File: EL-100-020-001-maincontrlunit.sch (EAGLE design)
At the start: 56 parts, among them T1 WS-TST-90°, U1 VNI4140K-32, U16 24AA256-I/SN, U19 ABS10-32.768KHZ-7-T, U2 VNI4140K-32, U8 MCP7940N-I/SN, U9 PMEG2005ET, X1 944-12-46-00, X2 944-12-46-00, X3 90G-14

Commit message: DIN-rail-controller
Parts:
- removed D5: SM15T39A, strasys_standard:SM15T39A
- removed OC8: TCMT1106, strasys_standard:TCMT1106
- added C11, C12, C13, C14, C15, C16, C17, C18, C23, C24, C25, C26, C31, C32, C33, C34, C64: 10nF, Kemet_By_element14_1:C0805C103K1RACTU
- added C19, C20, C21, C22, C27, C28, C29, C30, C35, C36, C37, C38, C43, C44, C45, C46, C47, C53, C54, C55, C56, C57, C58, C59, C60, C61, C62, C63, C65: 1000pF 1kV, supply2:C1206C102KDRACTU
- added C39, C40: 4.7nF, Kemet_By_element14_1:C0805F472K1RACAUTO
- added C41: 47UF, strasys_standard:EEE-FK1C470P-CASE-D
- added C42: 100nF, Kemet_By_element14_1:C0805C104K5RACTU
- added D1: (no value), strasys_standard:SMA6J33CA
- added L1: (no value), WE-CBF:WE-CBF-74279218_1206
- added R18, R19, R20, R33, R38, R39, R40, R46, R47, R48, R49, R57, R58, R59, R60, R62, R63, R64, R9: 1K Ohms, Vishay_By_element14_Batch_1:CRCW08051K00JNEA
- added R21, R22, R23, R24: 47K Ohms, Vishay_By_element14_Batch_1:CRCW080547K0JNEA
- added R25, R26, R27, R28, R29, R30, R31, R32, R34, R35, R36, R37, R41, R42, R43, R44, R45, R50, R51, R52, R53, R54, R55, R56, R61: 4.7K Ohms, Vishay_By_element14_Batch_1:CRCW08054K70JNEB
- added RV1, RV10, RV11, RV12, RV13, RV14, RV15, RV16, RV2, RV3, RV4, RV5, RV6, RV7, RV8, RV9: (no value), WE-VS:WE-VS-82550110_0805
- added U3: VNI4140K-32, strasys_standard:VNI4140K-32
- added X10, X11, X12, X9: S2L3.50/8/90G, strasys_standard:S2L3.50/8/90G
- added X4: 90G-14, strasys_standard:90G-14
- added X5, X6, X7, X8: Q-063209, con-erni:Q-063209
- C1: value 47µF -> 2.2uF; device strasys_standard:EEE-FK1H470P-CASE-E -> Kemet_By_element14_1:C1206C225K5RACTU; MF PANASONIC -> (none); MPN EEEFK1H470P -> (none); OC_FARNELL 9695931 -> (none)
- OC1, OC2, OC3, OC4, OC5, OC6, OC7: value TCMT1106 -> TCMT4106; device strasys_standard:TCMT1106 -> strasys_standard:TCMT4106; MF VISHAY -> (none)
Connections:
- new net ANA_1.1: C43.C2, RV1.2, X5.A1, X9.1
- new net ANA_1.2: C44.C2, RV2.2, X5.B1, X9.3
- new net ANA_1.3: C45.C2, RV3.2, X5.A2, X9.5
- new net ANA_1.4: C46.C2, RV4.2, X5.B2, X9.7
- new net ANA_2.1: C56.C2, RV9.2, X10.1, X6.A1
- new net ANA_2.2: C57.C2, RV10.2, X10.3, X6.B1
- new net ANA_2.3: C58.C2, RV11.2, X10.5, X6.A2
- new net ANA_2.4: C59.C2, RV12.2, X10.7, X6.B2
- new net ANA_3.1: C47.C2, RV5.2, X11.1, X7.A1
- new net ANA_3.2: C53.C2, RV6.2, X11.3, X7.B1
- new net ANA_3.3: C54.C2, RV7.2, X11.5, X7.A2
- new net ANA_3.4: C55.C2, RV8.2, X11.7, X7.B2
- new net ANA_4.1: C60.C2, RV13.2, X12.1, X8.A1
- new net ANA_4.2: C61.C2, RV14.2, X12.3, X8.B1
- new net ANA_4.3: C62.C2, RV15.2, X12.5, X8.A2
- new net ANA_4.4: C63.C2, RV16.2, X12.7, X8.B2
- new net IN_1: C22.C2, R45.1, X4.1
- new net IN_10: C37.C2, R55.1, X4.10
- new net IN_11: C36.C2, R54.1, X4.11
- new net IN_12: C35.C2, R53.1, X4.12
- new net IN_13: C65.C2, R61.1
- new net IN_2: C21.C2, R44.1, X4.2
- new net IN_3: C20.C2, R43.1, X4.3
- new net IN_4: C19.C2, R42.1, X4.4
- new net IN_5: C30.C2, R32.1, X4.5
- new net IN_6: C29.C2, R31.1, X4.6
- new net IN_7: C28.C2, R30.1, X4.7
- new net IN_8: C27.C2, R29.1, X4.8
- new net IN_9: C38.C2, R56.1, X4.9
- new net N$10: OC2.7, R8.2
- new net N$11: OC4.1, R9.2
- new net N$12: OC4.15, R21.1, U3.IN1
- new net N$13: OC4.13, R22.1, U3.IN2
- new net N$18: OC4.3, R18.2
- new net N$31: C24.C2, OC5.3, R30.2, R38.1
- new net N$32: C25.C2, OC5.5, R31.2, R39.1
- new net N$33: C26.C2, OC5.7, R32.2, R40.1
- new net N$34: C15.C2, OC3.1, R42.2, R46.1
- new net N$35: C31.C2, OC6.1, R53.2, R57.1
- new net N$36: C16.C2, OC3.3, R43.2, R47.1
- new net N$37: C32.C2, OC6.3, R54.2, R58.1
- new net N$38: C33.C2, OC6.5, R55.2, R59.1
- new net N$39: C34.C2, OC6.7, R56.2, R60.1
- new net N$40: C64.C2, OC7.1, R61.2, R62.1
- new net N$41: R63.2
- new net N$42: C17.C2, OC3.5, R44.2, R48.1
- new net N$43: OC7.7, R64.2
- new net N$49: C18.C2, OC3.7, R45.2, R49.1
- new net N$6: OC1.5, R3.2
- new net N$7: OC1.7, R4.2
- new net N$8: OC2.3, R6.2
- new net N$9: OC2.5, R7.2
- new net P8_27: R20.1, X2.27
- new net P8_28: R19.1, X2.28
- new net P8_29: R18.1, X2.29
- new net P8_30: R9.1, X2.30
- new net P8_39: OC5.10, R28.1, X2.39
- new net P8_40: OC5.12, R27.1, X2.40
- new net P8_41: OC5.14, R26.1, X2.41
- new net P8_42: OC5.16, R25.1, X2.42
- new net P8_43: OC6.10, R52.1, X2.43
- new net P8_44: OC6.12, R51.1, X2.44
- new net P8_45: OC6.14, R50.1, X2.45
- new net P8_46: OC6.16, R41.1, X2.46
- new net SYS5V_F: C41.1, C42.C2, L1.2, X5.A3, X6.A3, X7.A3, X8.A3
- net +24V: now also C1.C2, C39.C1, D1.2, OC1.10, OC1.12, OC1.14, OC1.16, OC2.10, OC2.12, OC2.16, OC4.10, OC4.12, OC4.16, U3.TAB, U3.VCC, X3.2; no longer C1.1, D5.C, OC1.4, OC2.4, OC3.4, OC4.4, OC5.4, OC6.4, OC7.4, OC8.4
- net +3.3V: now also R25.2, R26.2, R27.2, R28.2, R34.2, R35.2, R36.2, R37.2, R41.2, R50.2, R51.2, R52.2, X5.A4, X6.A4, X7.A4, X8.A4
- net 0V: now also C1.C1, C11.C1, C12.C1, C13.C1, C14.C1, C15.C1, C16.C1, C17.C1, C18.C1, C19.C1, C20.C1, C21.C1, C22.C1, C23.C1, C24.C1, C25.C1, C26.C1, C27.C1, C28.C1, C29.C1, C30.C1, C31.C1, C32.C1, C33.C1, C34.C1, C35.C1, C36.C1, C37.C1, C38.C1, C40.C2, C43.C1, C44.C1, C45.C1, C46.C1, C47.C1, C53.C1, C54.C1, C55.C1, C56.C1, C57.C1, C58.C1, C59.C1, C60.C1, C61.C1, C62.C1, C63.C1, C64.C1, C65.C1, D1.1, OC3.2, OC3.4, OC3.6, OC3.8, OC5.2, OC5.4, OC5.6, OC5.8, OC6.2, OC6.4, OC6.6, OC6.8, OC7.2, R21.2, R22.2, R23.2, R24.2, R33.2, R38.2, R39.2, R40.2, R46.2, R47.2, R48.2, R49.2, R57.2, R58.2, R59.2, R60.2, R62.2, U3.GND, X3.1; no longer C1.2, D5.A
- net AGND: now also RV1.1, RV10.1, RV11.1, RV12.1, RV13.1, RV14.1, RV15.1, RV16.1, RV2.1, RV3.1, RV4.1, RV5.1, RV6.1, RV7.1, RV8.1, RV9.1, X10.2, X10.4, X10.6, X10.8, X11.2, X11.4, X11.6, X11.8, X12.2, X12.4, X12.6, X12.8, X5.B3, X5.B4, X6.B3, X6.B4, X7.B3, X7.B4, X8.B3, X8.B4, X9.2, X9.4, X9.6, X9.8
- net AIN0: now also X5.A7
- net AIN1: now also X5.B7
- net AIN2: now also X5.A8
- net AIN3: now also X5.B8
- net AIN4: now also X5.A9
- net AIN5: now also X5.B9
- net AIN6: now also X5.A10
- net DGND: now also C41.2, C42.C1, OC1.4, OC1.6, OC1.8, OC2.4, OC2.6, OC2.8, OC3.11, OC3.13, OC3.15, OC3.9, OC4.4, OC4.6, OC4.8, OC5.11, OC5.13, OC5.15, OC5.9, OC6.11, OC6.13, OC6.15, OC6.9, OC7.6, OC7.8; no longer OC3.2, OC5.2, OC6.2, OC7.2, OC8.2
- net I2C1_SCL: now also X5.A6, X6.A6, X7.A6, X8.A6
- net I2C1_SDA: now also X5.A5, X6.A5, X7.A5, X8.A5
- net I2C2_SCL: now also X5.B6, X6.B6, X7.B6, X8.B6
- net I2C2_SDA: now also X5.B5, X6.B5, X7.B5, X8.B5
- net N$15: now also OC1.3; no longer OC2.1
- net N$16: now also OC4.11, R23.1, U3.IN3; no longer OC3.1, R3.2
- net N$17: now also OC4.9, R24.1, U3.IN4; no longer OC4.1, R4.2
- net N$19: now also OC1.15; no longer OC1.3
- net N$20: now also OC1.13; no longer OC2.3
- net N$21: now also OC1.11; no longer OC3.3
- net N$22: now also OC1.9; no longer OC4.3
- net N$23: now also OC2.1; no longer OC5.1
- net N$24: now also OC4.5, R19.2; no longer OC6.1, R6.2
- net N$25: now also OC4.7, R20.2; no longer OC7.1, R7.2
- net N$26: now also C23.C2, OC5.1, R29.2, R33.1; no longer OC8.1, R8.2
- net N$27: now also OC2.15; no longer OC5.3
- net N$28: now also OC2.13; no longer OC6.3
- net N$29: now also OC2.11; no longer OC7.3
- net N$30: now also OC2.9; no longer OC8.3
- net OUT_1: now also C6.C2, U1.OUT4, U1.OUT4_2, U1.OUT4_3, X3.14; no longer C3.C2, U1.OUT1, U1.OUT1_2, U1.OUT1_3, X3.1
- net OUT_10: now also C13.C2, U3.OUT3, U3.OUT3_2, U3.OUT3_3, X3.5; no longer X3.10
- net OUT_11: now also C12.C2, U3.OUT2, U3.OUT2_2, U3.OUT2_3, X3.4; no longer X3.11
- net OUT_12: now also C11.C2, U3.OUT1, U3.OUT1_2, U3.OUT1_3, X3.3; no longer X3.12
- net OUT_2: now also C5.C2, U1.OUT3, U1.OUT3_2, U1.OUT3_3, X3.13; no longer C4.C2, U1.OUT2, U1.OUT2_2, U1.OUT2_3, X3.2
- net OUT_3: now also C4.C2, U1.OUT2, U1.OUT2_2, U1.OUT2_3, X3.12; no longer C5.C2, U1.OUT3, U1.OUT3_2, U1.OUT3_3, X3.3
- net OUT_4: now also C3.C2, U1.OUT1, U1.OUT1_2, U1.OUT1_3, X3.11; no longer C6.C2, U1.OUT4, U1.OUT4_2, U1.OUT4_3, X3.4
- net OUT_5: now also C10.C2, U2.OUT4, U2.OUT4_2, U2.OUT4_3, X3.10; no longer C7.C2, U2.OUT1, U2.OUT1_2, U2.OUT1_3, X3.5
- net OUT_6: now also C9.C2, U2.OUT3, U2.OUT3_2, U2.OUT3_3, X3.9; no longer C8.C2, U2.OUT2, U2.OUT2_2, U2.OUT2_3, X3.6
- net OUT_7: now also C8.C2, U2.OUT2, U2.OUT2_2, U2.OUT2_3, X3.8; no longer C9.C2, U2.OUT3, U2.OUT3_2, U2.OUT3_3, X3.7
- net OUT_8: now also C7.C2, U2.OUT1, U2.OUT1_2, U2.OUT1_3, X3.7; no longer C10.C2, U2.OUT4, U2.OUT4_2, U2.OUT4_3, X3.8
- net OUT_9: now also C14.C2, U3.OUT4, U3.OUT4_2, U3.OUT4_3, X3.6; no longer X3.9
- net P8_15: now also OC3.16, R34.1
- net P8_16: now also OC3.14, R35.1
- net P8_17: now also OC3.12, R36.1
- net P8_18: now also OC3.10, R37.1
- net P9_14: now also R63.1
- net P9_15: now also R64.1
- net PE: now also C39.C2, C40.C1, X4.13, X4.14
- net SYS5V: now also L1.1
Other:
- note added: "24VDC"
- note added: "5VDC Filter"
- note added: "Anstatt Würth Multicomp: MCVZ0805M140AGT 14V / 35V Brake down"
- note added: "Controller power"
- note added: "ERROR"
- note added: "heartbeat"

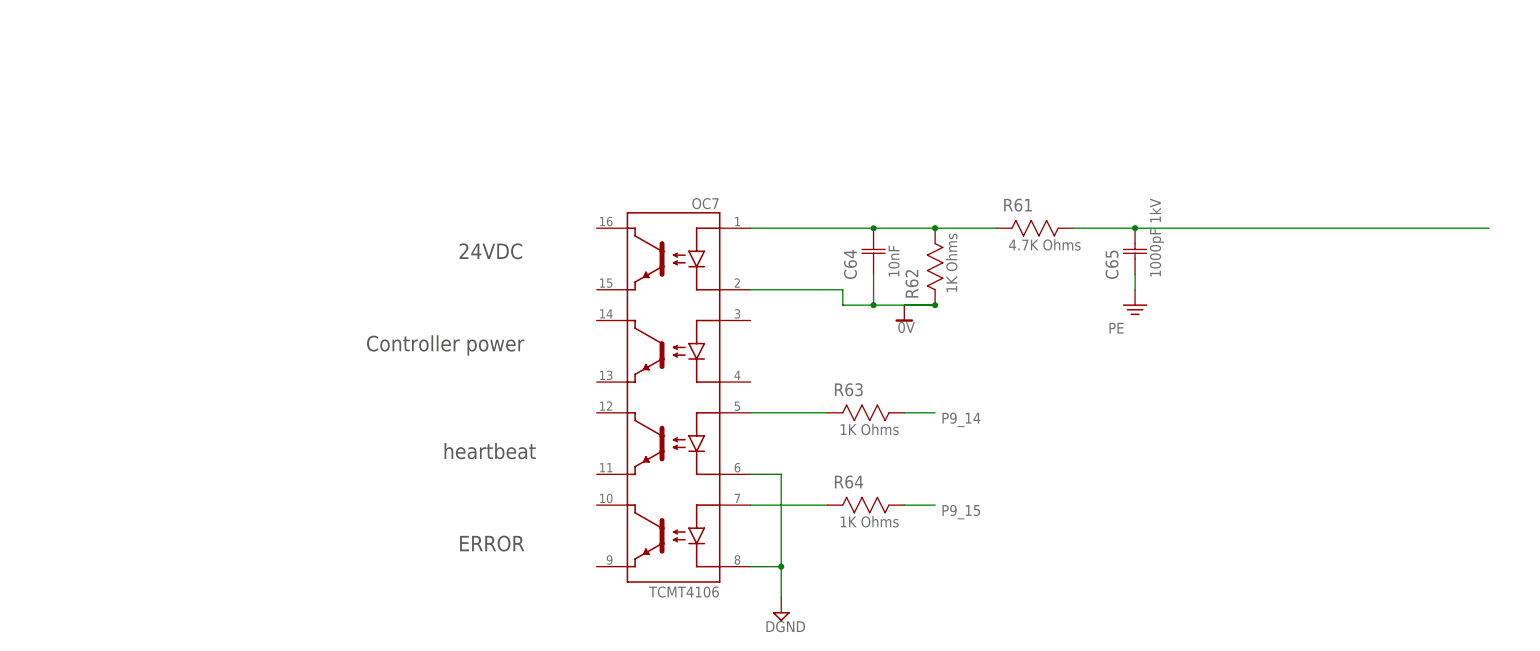
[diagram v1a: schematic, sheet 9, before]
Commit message: update new design
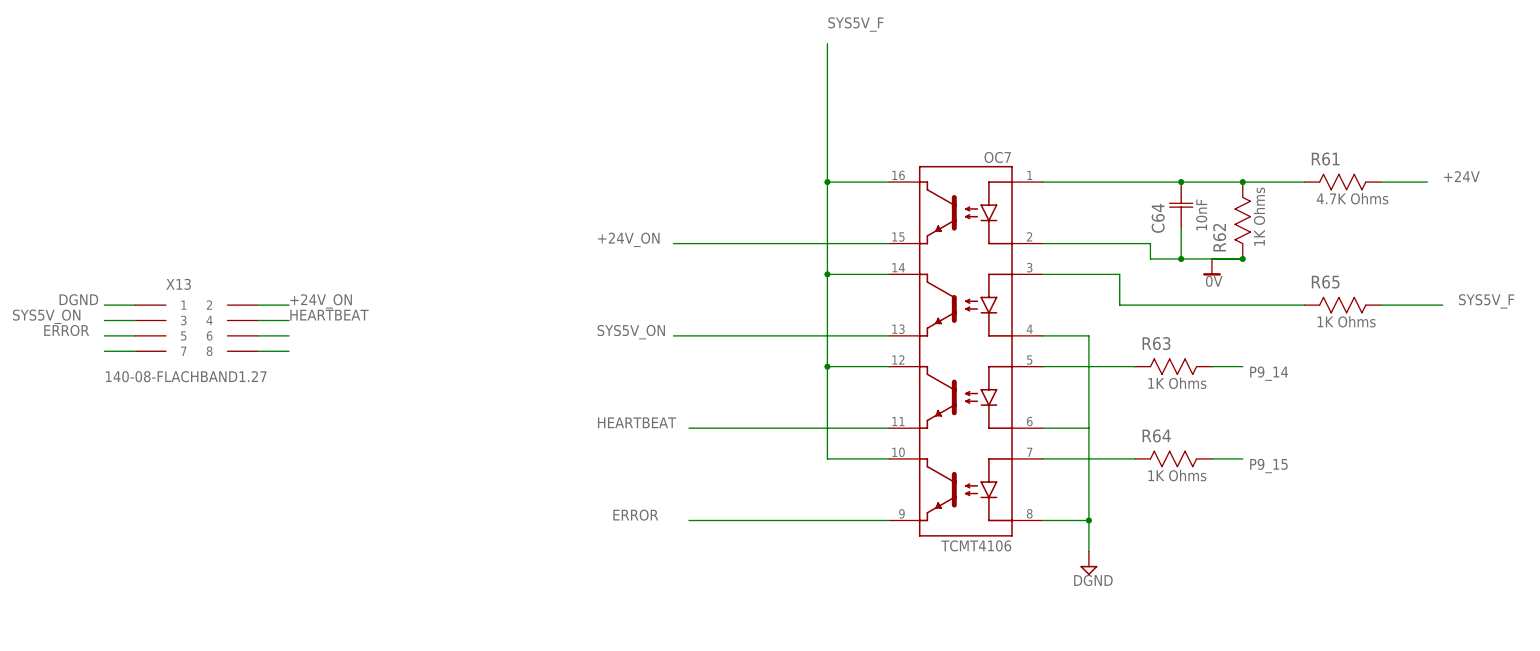
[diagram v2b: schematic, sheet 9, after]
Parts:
- removed C65: 1000pF 1kV, supply2:C1206C102KDRACTU
- removed S1: (no value), switch-dil:SD4-01
- added R65: 1K Ohms, Vishay_By_element14_Batch_1:CRCW08051K00JNEA
- added R66: 0 Ohms, Vishay_By_element14_Batch_1:CRCW12060000Z0EA
- added X13: 140-08-FLACHBAND1.27, strasys_standard:140-08-FLACHBAND1.27
- added X14: 944-12-2-00, strasys_standard:944-12-2-00
- C19, C20, C21, C22, C27, C28, C29, C30, C35, C36, C37, C38, C43, C44, C45, C46, C47, C53, C54, C55, C56, C57, C58, C59, C60, C61, C62, C63: value 1000pF 1kV -> 1000pF
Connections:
- removed net IN_13: C65.C2, R61.1
- new net +24V_ON: OC7.15, X13.2
- new net ERROR: OC7.9, X13.5
- new net HEARTBEAT: OC7.11, X13.4
- new net N$52: X13.7
- new net N$54: X13.6
- new net N$55: X13.8
- new net SYS5V_ON: OC7.13, X13.3
- net +24V: now also R61.1
- net 0V: no longer C19.C1, C20.C1, C21.C1, C22.C1, C27.C1, C28.C1, C29.C1, C30.C1, C35.C1, C36.C1, C37.C1, C38.C1, C65.C1
- net 24AA_WP: now also X14.2; no longer S1.1
- net AGND: now also R66.2
- net DGND: now also OC7.4, R66.1, X13.1, X14.1; no longer S1.2
- net N$41: now also OC7.5
- net PE: now also C19.C1, C20.C1, C21.C1, C22.C1, C27.C1, C28.C1, C29.C1, C30.C1, C35.C1, C36.C1, C37.C1, C38.C1
- net SYS5V_F: now also OC7.10, OC7.12, OC7.14, OC7.16, OC7.3, R65.1, R65.2
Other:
- note removed: "24VDC"
- note removed: "Controller power"
- note removed: "ERROR"
- note removed: "heartbeat"
- moved on the sheet: C64, OC7, R61, R62, R63, R64

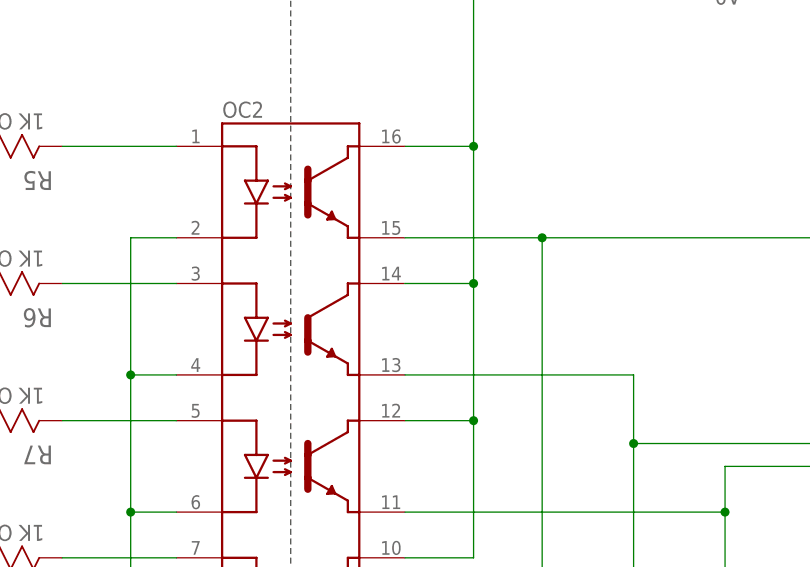
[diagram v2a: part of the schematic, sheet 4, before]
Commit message: update
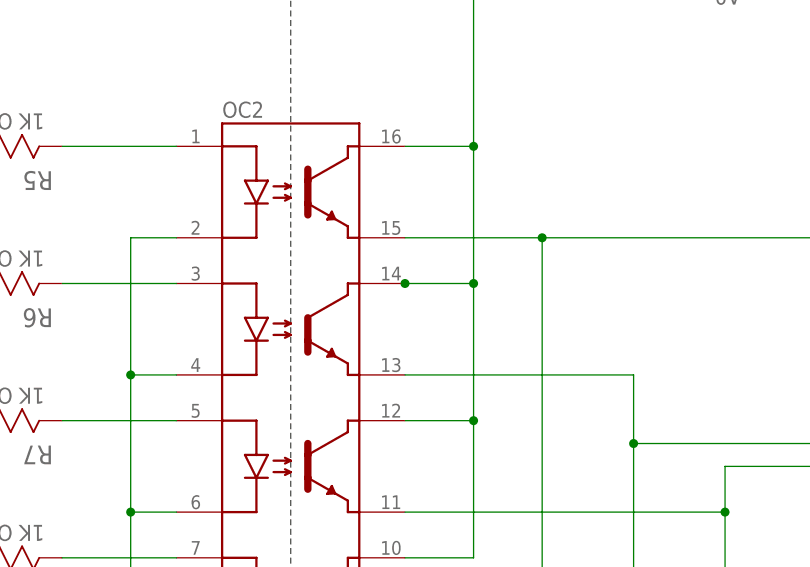
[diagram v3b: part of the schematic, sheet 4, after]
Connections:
- net +24V: now also OC2.14, OC4.14
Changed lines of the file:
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@@
 <wire x1="81.28" y1="119.38" x2="81.28" y2="104.14" width="0.1524" layer="91"/>
 <wire x1="81.28" y1="104.14" x2="81.28" y2="88.9" width="0.1524" layer="91"/>
+<junction x="81.28" y="119.38"/>
 <wire x1="73.66" y1="119.38" x2="81.28" y2="119.38" width="0.1524" layer="91"/>
-<junction x="81.28" y="119.38"/>
 <wire x1="81.28" y1="134.62" x2="81.28" y2="119.38" width="0.1524" layer="91"/>
 <wire x1="73.66" y1="134.62" x2="81.28" y2="134.62" width="0.1524" layer="91"/>
@@
 <pinref part="C1" gate="A" pin="C2"/>
 <pinref part="D1" gate="D$1" pin="2"/>
+<pinref part="OC2" gate="OC$1" pin="14"/>
+<junction x="73.66" y="119.38"/>
 </segment>
 </net>
@@
 <pinref part="U3" gate="A" pin="TAB"/>
 <wire x1="152.4" y1="172.72" x2="142.24" y2="172.72" width="0.1524" layer="91"/>
-<wire x1="78.74" y1="190.5" x2="86.36" y2="190.5" width="0.1524" layer="91"/>
-<wire x1="86.36" y1="220.98" x2="86.36" y2="205.74" width="0.1524" layer="91"/>
-<wire x1="86.36" y1="205.74" x2="86.36" y2="190.5" width="0.1524" layer="91"/>
+<label x="142.24" y="246.38" size="1.778" layer="95"/>
+</segment>
+<segment>
+<junction x="86.36" y="220.98"/>
+<pinref part="OC4" gate="OC$1" pin="14"/>
 <wire x1="78.74" y1="220.98" x2="86.36" y2="220.98" width="0.1524" layer="91"/>
-<junction x="86.36" y="220.98"/>
-<wire x1="86.36" y1="236.22" x2="86.36" y2="220.98" width="0.1524" layer="91"/>
+<pinref part="OC4" gate="OC$1" pin="16"/>
 <wire x1="78.74" y1="236.22" x2="86.36" y2="236.22" width="0.1524" layer="91"/>
 <junction x="86.36" y="236.22"/>
 <wire x1="86.36" y1="246.38" x2="86.36" y2="236.22" width="0.1524" layer="91"/>
-<pinref part="OC4" gate="OC$1" pin="16"/>
-<pinref part="OC4" gate="OC$1" pin="10"/>
+<wire x1="86.36" y1="236.22" x2="86.36" y2="220.98" width="0.1524" layer="91"/>
+<wire x1="86.36" y1="220.98" x2="86.36" y2="205.74" width="0.1524" layer="91"/>
 <pinref part="OC4" gate="OC$1" pin="12"/>
 <wire x1="78.74" y1="205.74" x2="86.36" y2="205.74" width="0.1524" layer="91"/>
 <junction x="86.36" y="205.74"/>
+<wire x1="86.36" y1="205.74" x2="86.36" y2="190.5" width="0.1524" layer="91"/>
+<wire x1="78.74" y1="190.5" x2="86.36" y2="190.5" width="0.1524" layer="91"/>
+<pinref part="OC4" gate="OC$1" pin="10"/>
 <label x="86.36" y="246.38" size="1.778" layer="95"/>
-<label x="142.24" y="246.38" size="1.778" layer="95"/>
 </segment>
 </net>
@@
 </sheet>
 </sheets>
+<errors>
+</errors>
 </schematic>
 </drawing>

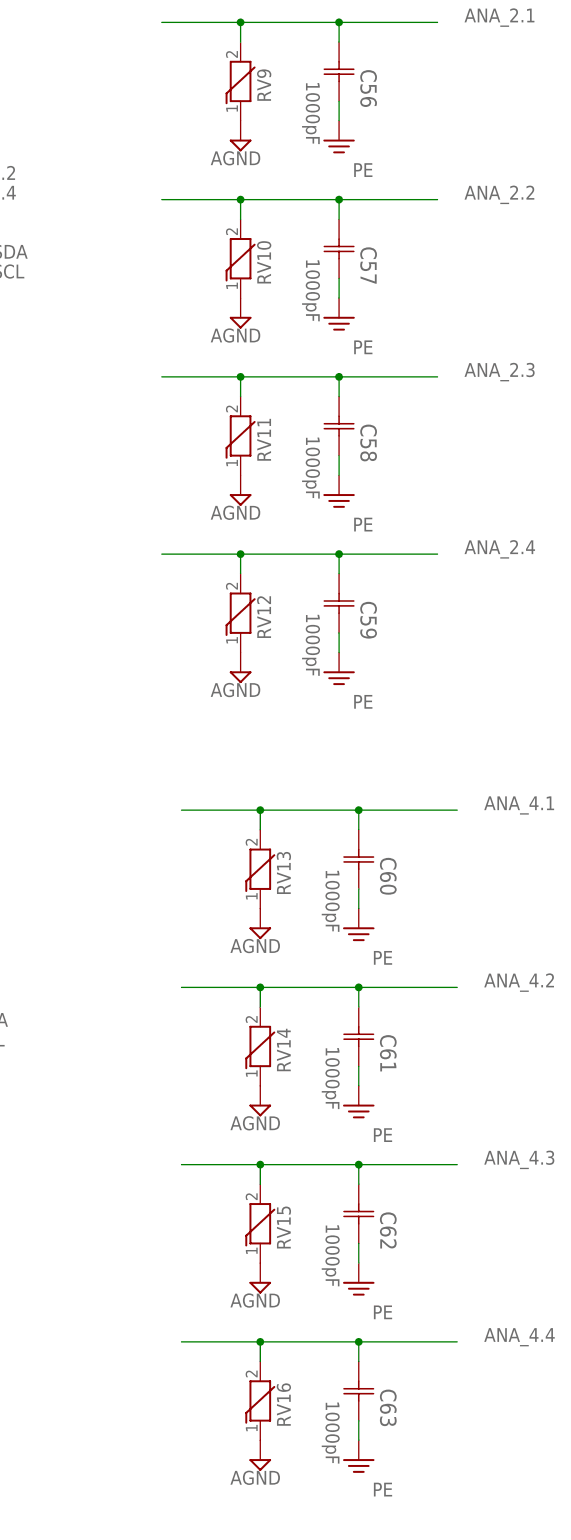
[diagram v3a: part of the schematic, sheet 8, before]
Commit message: new DIN rail hardware
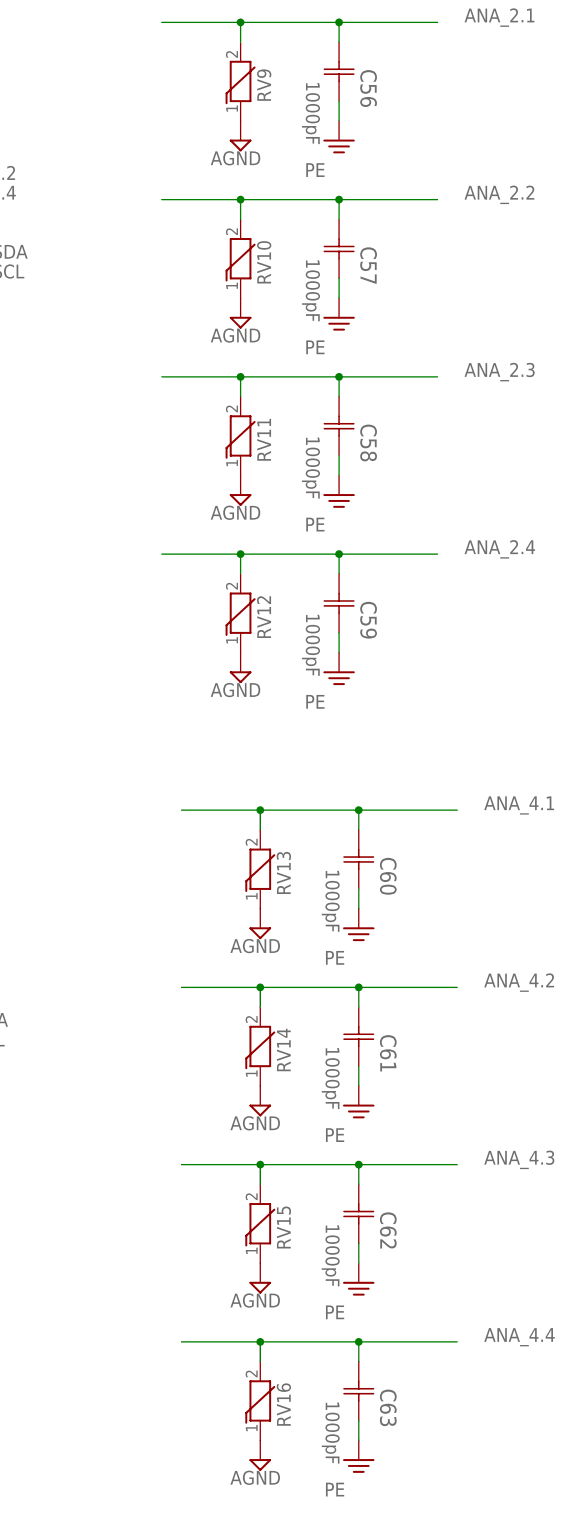
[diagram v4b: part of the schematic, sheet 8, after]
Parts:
- added R67, R68, R69, R70: 10K Ohms, Vishay_By_element14_Batch_1:CRCW080510K0JNEA
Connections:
- net 0V: no longer C43.C1, C44.C1, C45.C1, C46.C1, C47.C1, C53.C1, C54.C1, C55.C1, C56.C1, C57.C1, C58.C1, C59.C1, C60.C1, C61.C1, C62.C1, C63.C1
- net PE: now also C43.C1, C44.C1, C45.C1, C46.C1, C47.C1, C53.C1, C54.C1, C55.C1, C56.C1, C57.C1, C58.C1, C59.C1, C60.C1, C61.C1, C62.C1, C63.C1
